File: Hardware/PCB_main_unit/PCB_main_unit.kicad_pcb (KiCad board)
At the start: 4 copper layers, 60 x 60 mm, 49 parts, among them J1 Conn_01x03, J10 Conn_01x03, J11 Conn_01x03, J12 Conn_01x04, J13 Conn_01x07, J14 Conn_ST_STDC14, J15 Conn_01x03, J16 Conn_01x02, J2 Conn_01x03, J3 Conn_01x03, J4 Conn_01x03, J5 Conn_01x03, J6 Conn_01x03, J7 Conn_01x03, J8 Conn_01x03, J9 Conn_01x06, SW1 SW_SPDT, U2 STM32G474RETx, U3 AZ1117-3.3

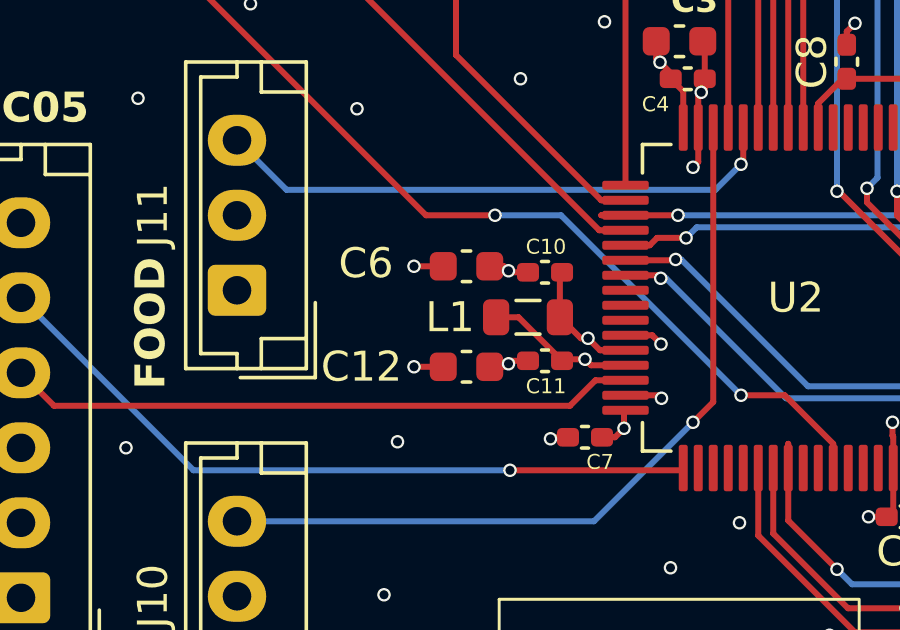
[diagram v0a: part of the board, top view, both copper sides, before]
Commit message: minor changes
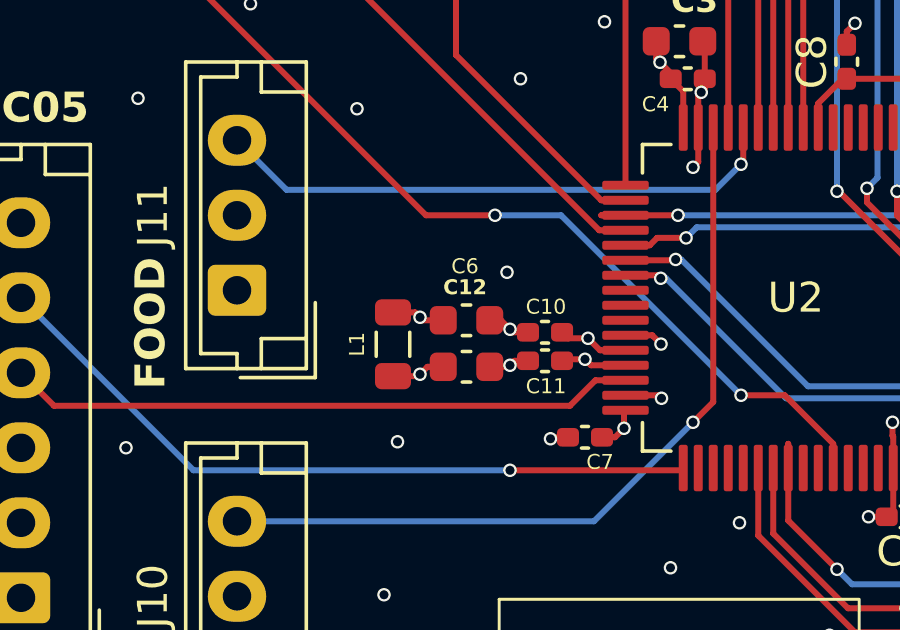
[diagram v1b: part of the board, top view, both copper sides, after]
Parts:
- moved L1 4.59 mm to (134.4, 110.3), turned to -90 degrees
- moved C10 2.00 mm to (139.5, 109.9)
- moved C6 1.80 mm to (136.8, 109.5)
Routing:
- net +3.3V: track 48.4 -> 45.4 mm
- net GND: vias 59 -> 60
